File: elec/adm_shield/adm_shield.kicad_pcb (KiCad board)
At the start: 2 copper layers, 35 parts

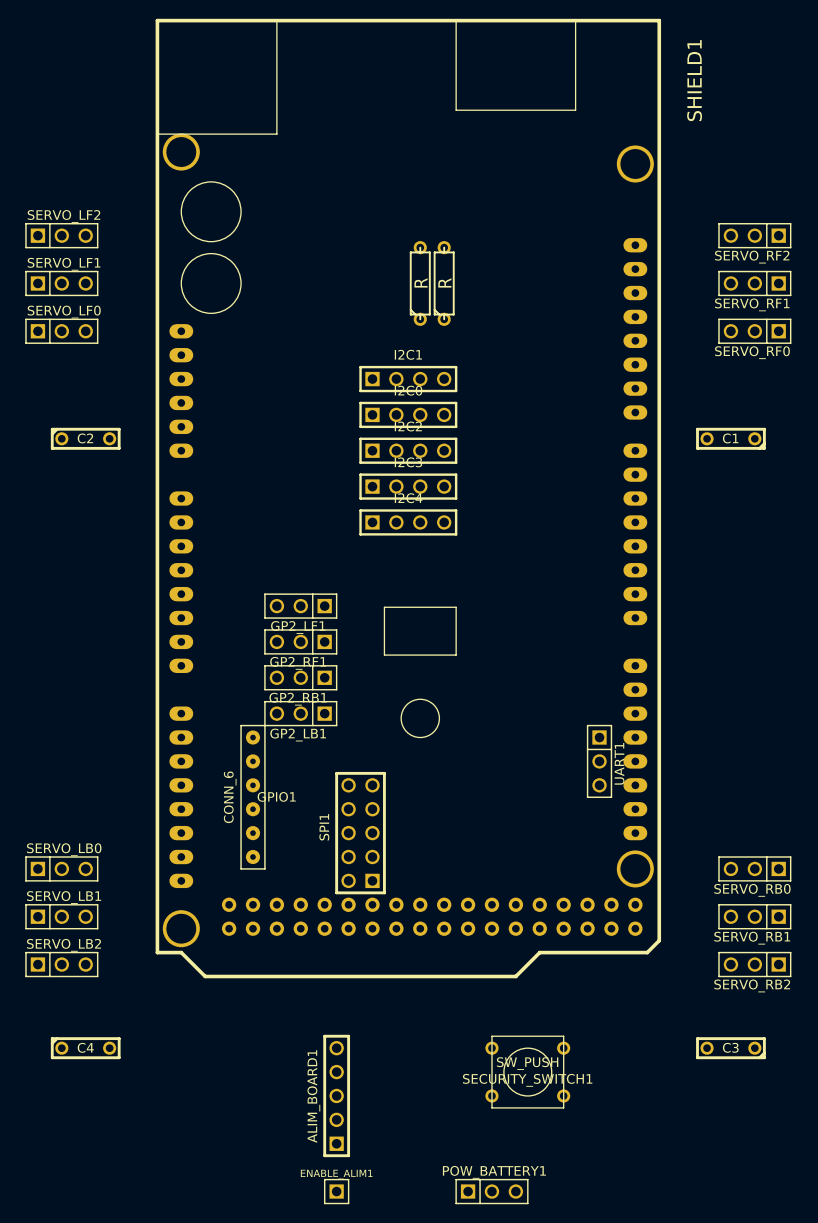
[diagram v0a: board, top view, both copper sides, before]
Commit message: PCB almost finished !
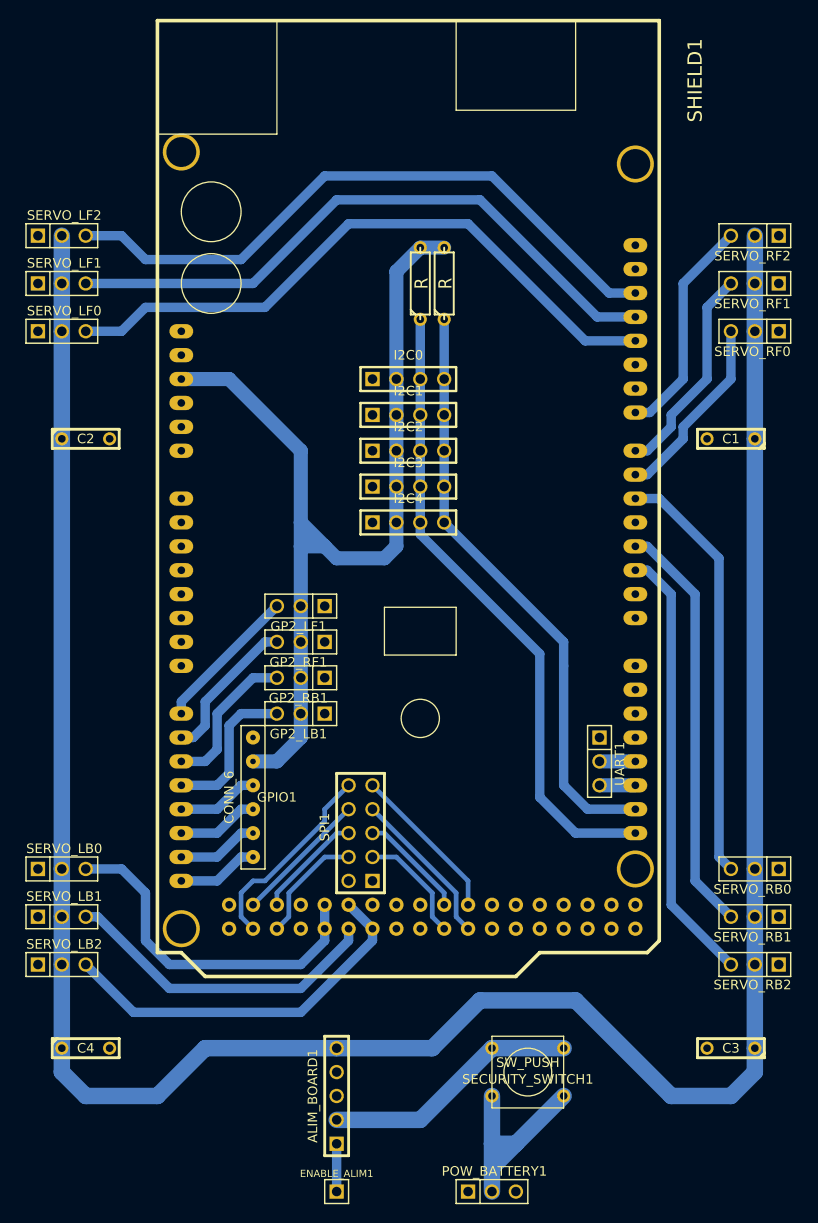
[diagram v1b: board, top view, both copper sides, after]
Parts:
- moved I2C0 3.81 mm to (222.2, 105.4)
- moved I2C1 3.81 mm to (222.2, 109.2)
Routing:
- net /ALIM/POW_5V: track 0.00 -> 262.0 mm
- net /ARDUINO/LOG_5V: track 0.00 -> 102.6 mm
- net /LEG_LF/PWM2: track 0.00 -> 68.3 mm
- net /LEG_LF/PWM0: track 0.00 -> 68.3 mm
- net /ARDUINO/SCL: track 0.00 -> 67.8 mm
- net /LEG_LF/PWM1: track 0.00 -> 67.3 mm
- net /ARDUINO/SDA: track 0.00 -> 63.5 mm
- net /LEG_RB/PWM2: track 0.00 -> 46.9 mm
- net /LEG_RB/PWM0: track 0.00 -> 45.1 mm
- net /LEG_RB/PWM1: track 0.00 -> 44.3 mm
- net /LEG_LB/PWM2: track 0.00 -> 40.6 mm
- net /LEG_LB/PWM0: track 0.00 -> 37.4 mm
- net /LEG_LB/PWM1: track 0.00 -> 34.5 mm
- net /ALIM/BAT: track 0.00 -> 27.3 mm
- net /LEG_RF/PWM2: track 0.00 -> 23.9 mm
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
